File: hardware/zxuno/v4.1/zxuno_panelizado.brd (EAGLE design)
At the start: 190 x 150 mm, 414 parts, among them T1 BC846, T2 BC846, T3 BC846, T4 BC846, U1 6SLX9TQG144, U10 FLASH-SPI-25XXSMD1, U11 3.3V, U12 1.2V, U13 AD724, U14 50MHz, U15 6SLX9TQG144, U17 FLASH-SPI-25XXSMD1, U18 3.3V, U19 1.2V, U2 FLASH-SPI-25XXSMD1, U20 AD724, U21 50MHz, U22 6SLX9TQG144, U24 FLASH-SPI-25XXSMD1, U25 3.3V, U26 1.2V, U27 AD724, U28 50MHz, U4 AD724, U5 50MHz, U6 3.3V, U7 1.2V, U8 6SLX9TQG144, Y1 3.58M, Y2 4.43M, Y3 3.58M, Y4 4.43M, Y5 3.58M, Y6 4.43M, Y7 3.58M, Y8 4.43M

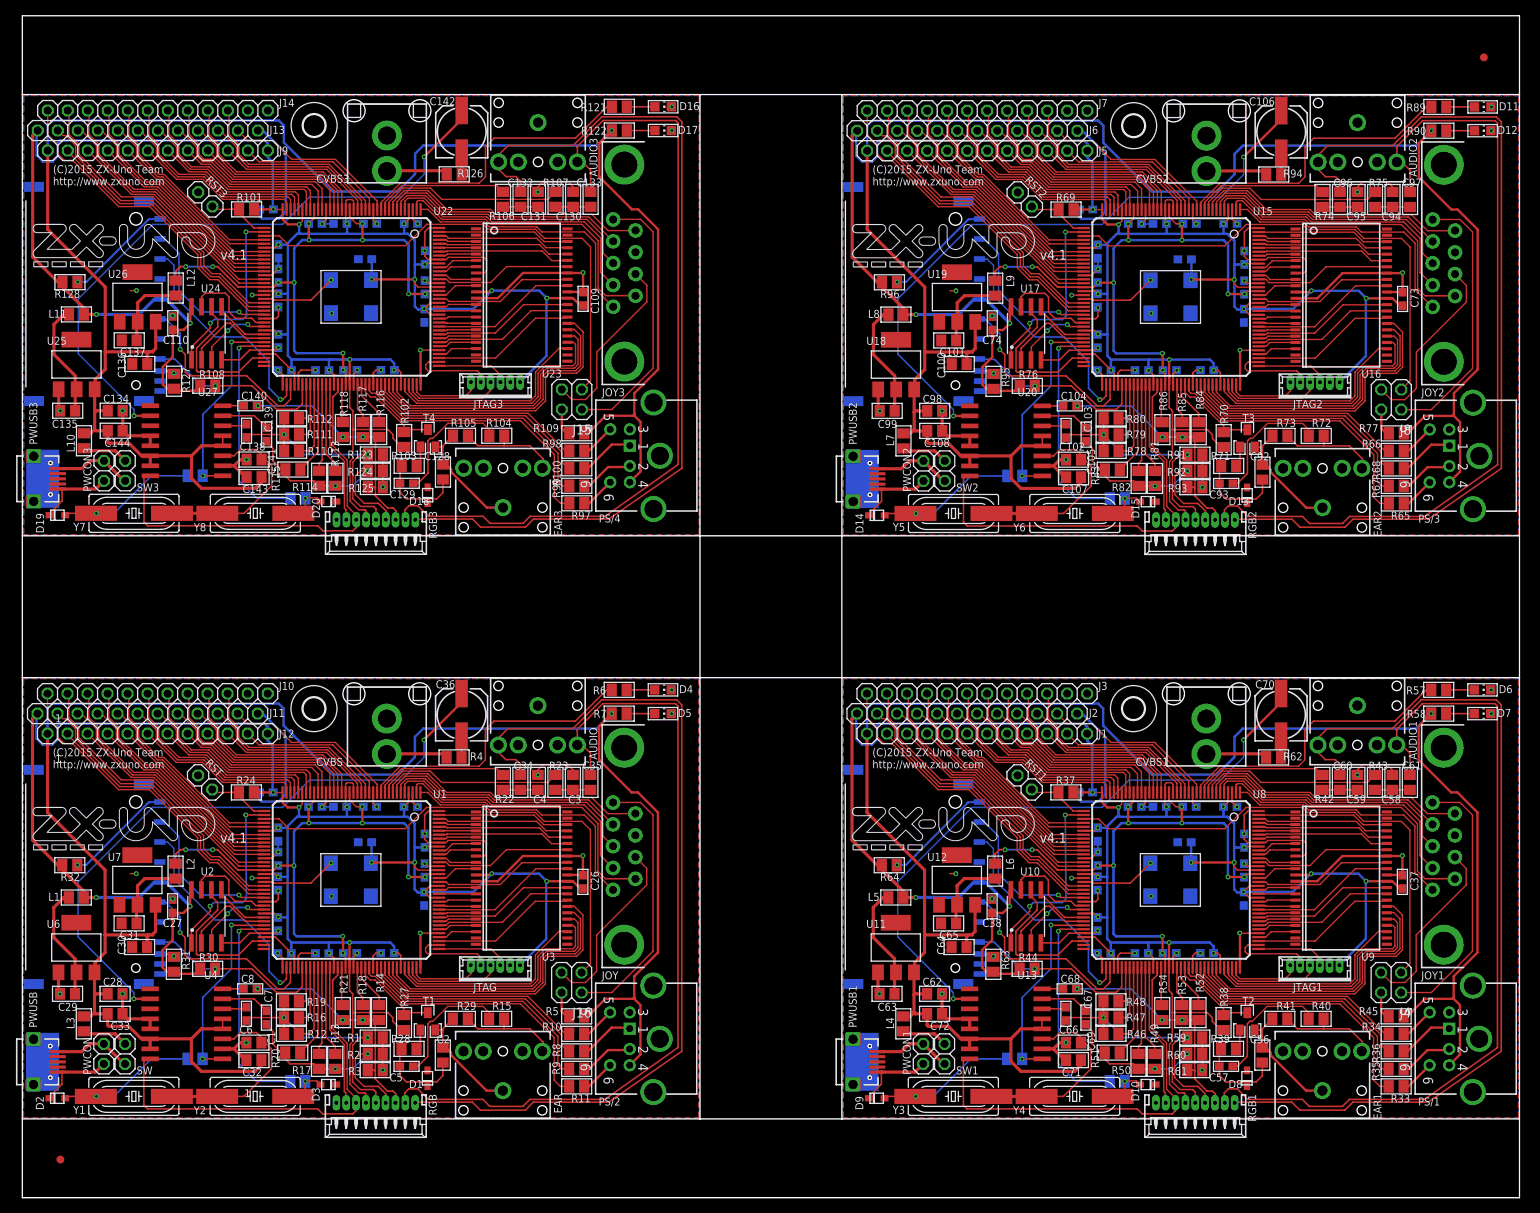
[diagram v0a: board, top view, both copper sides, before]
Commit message: Vacío panelizado
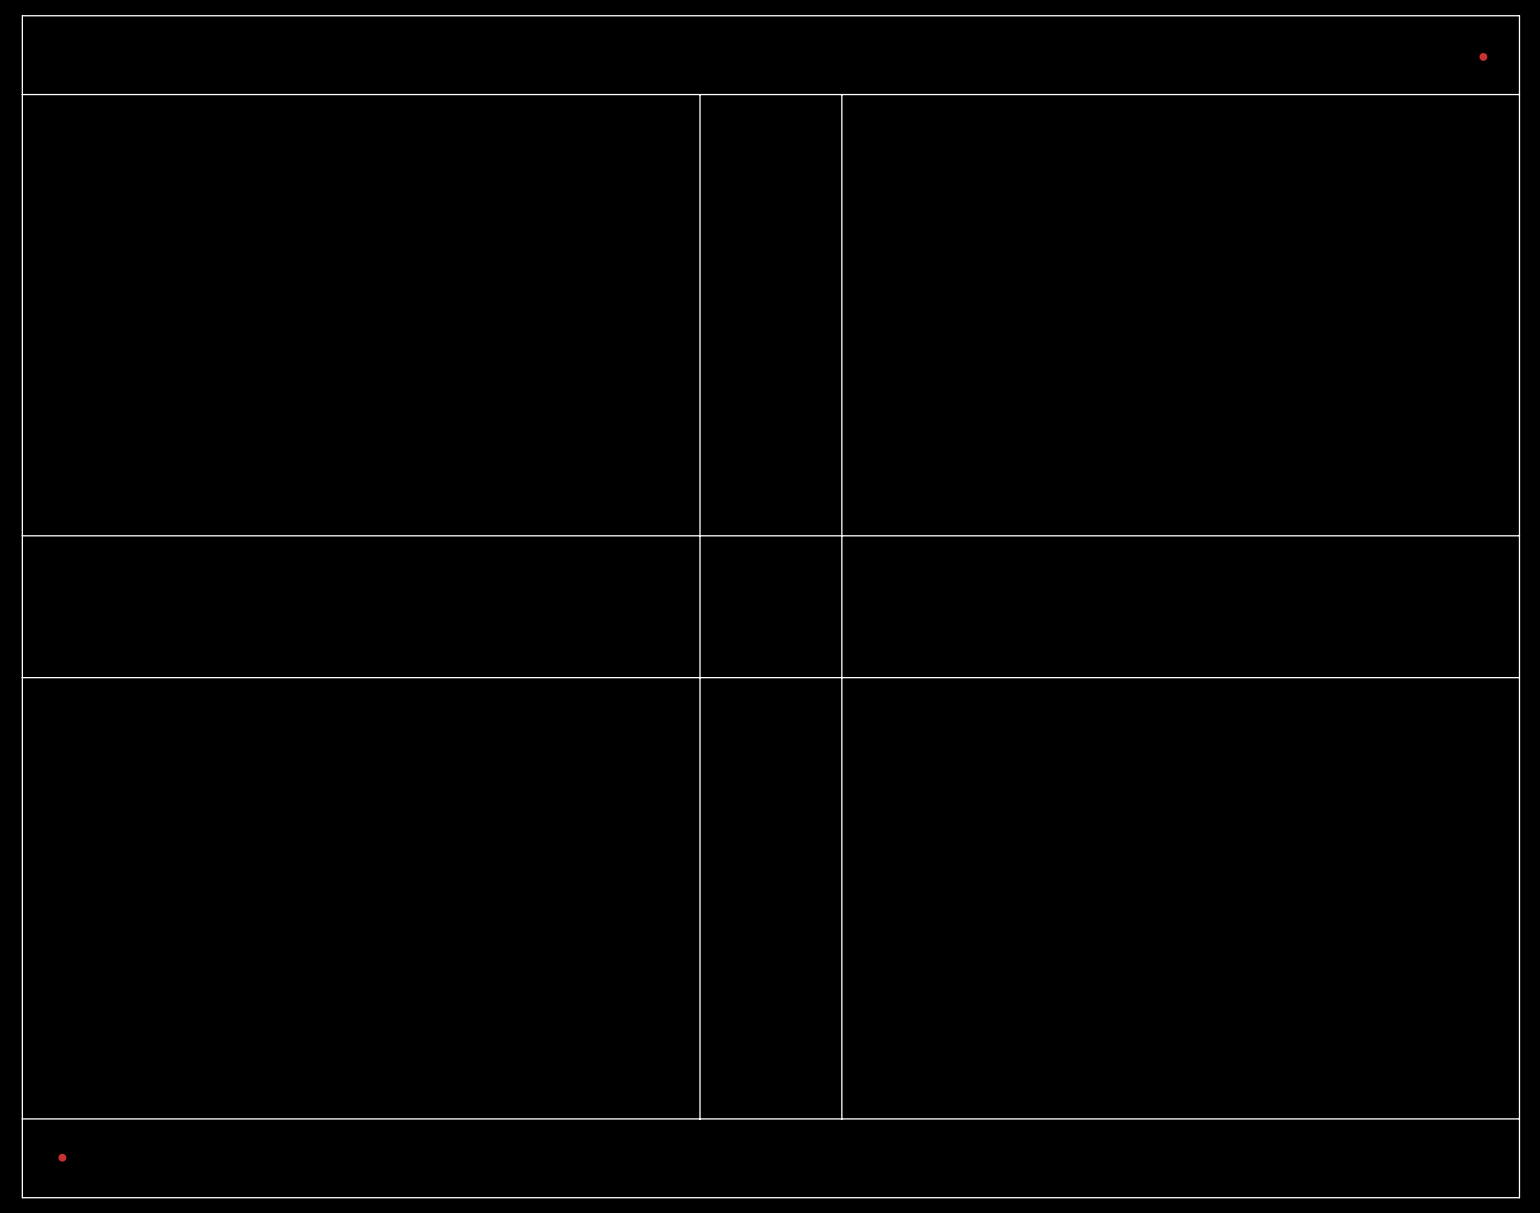
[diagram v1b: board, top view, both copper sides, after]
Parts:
- removed AUDIO, AUDIO1, AUDIO2, AUDIO3: Audio, SparkFun-Connectors:AUDIO-JACK
- removed C1, C105, C141, C69: 7.5pF, rcl:C0805
- removed C10, C102, C103, C104, C109, C11, C110, C111, C112, C113, C114, C115, C116, C117, C118, C119, C12, C120, C121, C122, C123, C124, C125, C126, C127, C129, C13, C138, C139, C14, C140, C15, C16, C17, C18, C19, C20, C21, C22, C23, C24, C25, C26, C27, C37, C38, C39, C40, C41, C42, C43, C44, C45, C46, C47, C48, C49, C5, C50, C51, C52, C53, C54, C55, C57, C6, C66, C67, C68, C7, C73, C74, C75, C76, C77, C78, C79, C8, C80, C81, C82, C83, C84, C85, C86, C87, C88, C89, C9, C90, C91, C93: 100nF, rcl:C0603
- removed C100, C101, C107, C108, C132, C133, C134, C135, C136, C137, C143, C144, C28, C29, C30, C31, C32, C33, C34, C35, C60, C61, C62, C63, C64, C65, C71, C72, C96, C97, C98, C99: 10uF, rcl:C0805
- removed C106, C142, C36, C70: 220uF, rcl:153CLV-0605
- removed C128, C130, C131, C2, C3, C4, C56, C58, C59, C92, C94, C95: 10nF, rcl:C0805
- removed CVBS, CVBS1, CVBS2, CVBS3: RCA, uzebox:RCA
- removed D1, D10, D13, D14, D15, D18, D19, D2, D20, D3, D8, D9: (no value), adafruit:SOD-323F
- removed D11, D12, D16, D17, D4, D5, D6, D7: (no value), led:CHIP-LED0805
- removed EAR, EAR1, EAR2, EAR3: EAR, SparkFun-Connectors:AUDIO-JACK
- removed H1, H2, H3, H4: MOUNT-HOLE2.8, holes:2,8
- removed J1, J10, J11, J12, J13, J14, J2, J3, J5, J6, J7, J9: (no value), pinhead:1X12
- removed J15, J16, J4, J8: (no value), pinhead:2X02
- removed JOY, JOY1, JOY2, JOY3: (no value), SparkFun-Connectors:DB9_MALE
- removed JTAG, JTAG1, JTAG2, JTAG3: JTAG, con-molex:53047-06
- removed L1, L10, L11, L12, L2, L3, L4, L5, L6, L7, L8, L9: (no value), rcl:M0805
- removed PS/1, PS/2, PS/3, PS/4: PS/2 Keyb, ZX_UNO_0_14:DINC/MIN_TM/6_1PRIMARY
- removed PWCON, PWCON1, PWCON2, PWCON3, RST, RST1, RST2, RST3, SW, SW1, SW2, SW3: (no value), pinhead:1X02
- removed PWUSB, PWUSB1, PWUSB2, PWUSB3: MICROUSB, zxuno_rev_mcleod:MICRO_USB_1PRIMARY
- removed R1, R123, R124, R125, R126, R2, R3, R4, R59, R60, R61, R62, R91, R92, R93, R94: 75, rcl:M0805
- removed R10, R100, R104, R109, R11, R110, R113, R116, R12, R121, R122, R13, R14, R15, R33, R34, R35, R36, R40, R45, R46, R49, R5, R52, R57, R58, R6, R65, R66, R67, R68, R7, R72, R77, R78, R8, R81, R84, R89, R9, R90, R97, R98, R99: 510, rcl:M0805
- removed R101, R106, R107, R112, R115, R118, R19, R20, R21, R22, R23, R24, R37, R42, R43, R48, R51, R54, R69, R74, R75, R80, R83, R86: 2K, rcl:M0805
- removed R102, R103, R105, R108, R119, R120, R127, R128, R25, R26, R27, R28, R29, R30, R31, R32, R38, R39, R41, R44, R55, R56, R63, R64, R70, R71, R73, R76, R87, R88, R95, R96: 10K, rcl:M0805
- removed R111, R114, R117, R16, R17, R18, R47, R50, R53, R79, R82, R85: 1K, rcl:M0805
- removed RGB, RGB1, RGB2, RGB3: RGB, con-molex:53048-09
- removed SDCARD, SDCARD1, SDCARD2, SDCARD3: (no value), zxuno_rev_mcleod:SDCMF-10915W010
- removed T1, T2, T3, T4: BC846, transistor:SOT23
- removed U1, U15, U22, U8: 6SLX9TQG144, xilinx_devices_V6:TQ144
- removed U10, U17, U2, U24: FLASH-SPI-25XXSMD1, GadgetFactory:SO08-EIAJ
- removed U11, U18, U25, U6: 3.3V, burr-brown:SOT223
- removed U12, U19, U26, U7: 1.2V, burr-brown:SOT223
- removed U13, U20, U27, U4: AD724, ad725:SO16W
- removed U14, U21, U28, U5: 50MHz, ZX_UNO_0_15:SM/OSC_1PRIMARY
- removed U16, U23, U3, U9: (no value), GadgetFactory:TSOP44-II
- removed Y1, Y3, Y5, Y7: 3.58M, crystal:HC49UP
- removed Y2, Y4, Y6, Y8: 4.43M, crystal:HC49UP
- moved E$1 0.35 mm to (5.08, 5.08)
- moved E$2 0.08 mm to (185.4, 144.8)
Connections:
- removed net 1.2V: C10.2, C11.2, C12.2, C13.2, C9.2, L2.2, U1.P128, U1.P19, U1.P28, U1.P52, U1.P89
- removed net 1.2V1: C39.2, C40.2, C41.2, C42.2, C43.2, L6.2, U8.P128, U8.P19, U8.P28, U8.P52, U8.P89
- removed net 1.2V2: C75.2, C76.2, C77.2, C78.2, C79.2, L9.2, U15.P128, U15.P19, U15.P28, U15.P52, U15.P89
- removed net 1.2V3: C111.2, C112.2, C113.2, C114.2, C115.2, L12.2, U22.P128, U22.P19, U22.P28, U22.P52, U22.P89
- removed net 3.3V: C14.2, C15.2, C16.2, C17.2, C18.2, C19.2, C20.2, C21.2, C22.2, C23.2, C24.2, C25.2, C26.1, C27.2, J11.1, J12.12, JTAG.1, L1.2, R24.2, R27.2, R30.1, R31.2, R32.2, RGB.4, SDCARD.4, U1.P103, U1.P122, U1.P125, U1.P129, U1.P135, U1.P18, U1.P20, U1.P31, U1.P36, U1.P4, U1.P42, U1.P53, U1.P63, U1.P69, U1.P76, U1.P86, U1.P90, U2.8, U3.11, U3.33, U5.4
- removed net 3.3V1: C37.1, C38.2, C44.2, C45.2, C46.2, C47.2, C48.2, C49.2, C50.2, C51.2, C52.2, C53.2, C54.2, C55.2, J1.12, J2.1, JTAG1.1, L5.2, R37.2, R38.2, R44.1, R63.2, R64.2, RGB1.4, SDCARD1.4, U10.8, U14.4, U8.P103, U8.P122, U8.P125, U8.P129, U8.P135, U8.P18, U8.P20, U8.P31, U8.P36, U8.P4, U8.P42, U8.P53, U8.P63, U8.P69, U8.P76, U8.P86, U8.P90, U9.11, U9.33
- removed net 3.3V2: C73.1, C74.2, C80.2, C81.2, C82.2, C83.2, C84.2, C85.2, C86.2, C87.2, C88.2, C89.2, C90.2, C91.2, J5.12, J6.1, JTAG2.1, L8.2, R69.2, R70.2, R76.1, R95.2, R96.2, RGB2.4, SDCARD2.4, U15.P103, U15.P122, U15.P125, U15.P129, U15.P135, U15.P18, U15.P20, U15.P31, U15.P36, U15.P4, U15.P42, U15.P53, U15.P63, U15.P69, U15.P76, U15.P86, U15.P90, U16.11, U16.33, U17.8, U21.4
- removed net 3.3V3: C109.1, C110.2, C116.2, C117.2, C118.2, C119.2, C120.2, C121.2, C122.2, C123.2, C124.2, C125.2, C126.2, C127.2, J13.1, J9.12, JTAG3.1, L11.2, R101.2, R102.2, R108.1, R127.2, R128.2, RGB3.4, SDCARD3.4, U22.P103, U22.P122, U22.P125, U22.P129, U22.P135, U22.P18, U22.P20, U22.P31, U22.P36, U22.P4, U22.P42, U22.P53, U22.P63, U22.P69, U22.P76, U22.P86, U22.P90, U23.11, U23.33, U24.8, U28.4
- removed net 5V: C28.1, C30.1, C32.2, C33.2, J12.1, L3.2, PS/2.4, R5.1, R7.2, U4.14, U4.15, U4.4, U4.5, U6.3, U7.3
- removed net 5V1: C62.1, C64.1, C71.2, C72.2, J1.1, L4.2, PS/1.4, R45.1, R58.2, U11.3, U12.3, U13.14, U13.15, U13.4, U13.5
- removed net 5V2: C100.1, C107.2, C108.2, C98.1, J5.1, L7.2, PS/3.4, R77.1, R90.2, U18.3, U19.3, U20.14, U20.15, U20.4, U20.5
- removed net 5V3: C134.1, C136.1, C143.2, C144.2, J9.1, L10.2, PS/4.4, R109.1, R122.2, U25.3, U26.3, U27.14, U27.15, U27.4, U27.5
- removed net AUDIO_LEFT: R22.2, U1.P10
- removed net AUDIO_LEFT1: R42.2, U8.P10
- removed net AUDIO_LEFT2: R74.2, U15.P10
- removed net AUDIO_LEFT3: R106.2, U22.P10
- removed net AUDIO_RIGHT: R23.2, U1.P9
- removed net AUDIO_RIGHT1: R43.2, U8.P9
- removed net AUDIO_RIGHT2: R75.2, U15.P9
- removed net AUDIO_RIGHT3: R107.2, U22.P9
- removed net B: C8.2, R14.1, R18.1, R21.1, R3.1, RGB.7
- removed net B0: R21.2, U1.P88
- removed net B1: R18.2, U1.P92
- removed net B10: C104.2, R84.1, R85.1, R86.1, R93.1, RGB2.7
- removed net B11: R118.2, U22.P88
- removed net B12: R117.2, U22.P92
- removed net B13: R116.2, U22.P93
- removed net B14: C140.2, R116.1, R117.1, R118.1, R125.1, RGB3.7
- removed net B2: R14.2, U1.P93
- removed net B3: R54.2, U8.P88
- removed net B4: R53.2, U8.P92
- removed net B5: R52.2, U8.P93
- removed net B6: C68.2, R52.1, R53.1, R54.1, R61.1, RGB1.7
- removed net B7: R86.2, U15.P88
- removed net B8: R85.2, U15.P92
- removed net B9: R84.2, U15.P93
- removed net CLK: U1.P55, U5.3
- removed net CLK1: U14.3, U8.P55
- removed net CLK2: U15.P55, U21.3
- removed net CLK3: U22.P55, U28.3
- removed net CSYNC: RGB.3, U1.P87, U4.16
- removed net CSYNC1: RGB1.3, U13.16, U8.P87
- removed net CSYNC2: RGB2.3, U15.P87, U20.16
- removed net CSYNC3: RGB3.3, U22.P87, U27.16
- removed net EAR: R27.1, T1.3, U1.P94
- removed net EAR1: R38.1, T2.3, U8.P94
- removed net EAR2: R70.1, T3.3, U15.P94
- removed net EAR3: R102.1, T4.3, U22.P94
- removed net EXT1: J1.2, U8.P57
- removed net EXT10: J12.3, U1.P50
- removed net EXT100: J9.5, U22.P43
- removed net EXT101: J13.5, U22.P41
- removed net EXT102: J14.5, U22.P40
- removed net EXT103: J9.6, U22.P35
- removed net EXT104: J13.6, U22.P34
- removed net EXT105: J14.6, U22.P33
- removed net EXT106: J9.7, U22.P32
- removed net EXT107: J13.7, U22.P30
- removed net EXT108: J14.7, U22.P29
- removed net EXT109: J9.8, U22.P27
- removed net EXT11: J11.3, U1.P48
- removed net EXT110: J13.8, U22.P26
- removed net EXT111: J14.8, U22.P24
- removed net EXT112: J9.9, U22.P23
- removed net EXT113: J13.9, U22.P22
- removed net EXT114: J14.9, U22.P21
- removed net EXT115: J9.10, U22.P17
- removed net EXT116: J13.10, U22.P16
- removed net EXT117: J14.10, U22.P15
- removed net EXT118: J9.11, U22.P14
- removed net EXT119: J13.11, U22.P12
- removed net EXT12: J10.3, U1.P47
- removed net EXT120: J14.1, U22.P58
- removed net EXT13: J12.4, U1.P46
- removed net EXT14: J11.4, U1.P45
- removed net EXT15: J10.4, U1.P44
- removed net EXT16: J12.5, U1.P43
- removed net EXT17: J11.5, U1.P41
- removed net EXT18: J10.5, U1.P40
- removed net EXT19: J12.6, U1.P35
- removed net EXT2: J2.2, U8.P56
- removed net EXT20: J11.6, U1.P34
- removed net EXT21: J10.6, U1.P33
- removed net EXT22: J12.7, U1.P32
- removed net EXT23: J11.7, U1.P30
- removed net EXT24: J10.7, U1.P29
- removed net EXT25: J12.8, U1.P27
- removed net EXT26: J11.8, U1.P26
- removed net EXT27: J10.8, U1.P24
- removed net EXT28: J12.9, U1.P23
- removed net EXT29: J11.9, U1.P22
- removed net EXT3: J3.2, U8.P51
- removed net EXT30: J10.9, U1.P21
- removed net EXT31: J12.10, U1.P17
- removed net EXT32: J11.10, U1.P16
- removed net EXT33: J10.10, U1.P15
- removed net EXT34: J12.11, U1.P14
- removed net EXT35: J11.11, U1.P12
- removed net EXT36: J3.3, U8.P47
- removed net EXT37: J1.4, U8.P46
- removed net EXT38: J2.4, U8.P45
- removed net EXT39: J3.4, U8.P44
- removed net EXT4: J1.3, U8.P50
- removed net EXT40: J1.5, U8.P43
- removed net EXT41: J2.5, U8.P41
- removed net EXT42: J3.5, U8.P40
- removed net EXT43: J1.6, U8.P35
- removed net EXT44: J2.6, U8.P34
- removed net EXT45: J3.6, U8.P33
- removed net EXT46: J1.7, U8.P32
- removed net EXT47: J2.7, U8.P30
- removed net EXT48: J3.7, U8.P29
- removed net EXT49: J1.8, U8.P27
- removed net EXT5: J2.3, U8.P48
- removed net EXT50: J2.8, U8.P26
- removed net EXT51: J3.8, U8.P24
- removed net EXT52: J1.9, U8.P23
- removed net EXT53: J2.9, U8.P22
- removed net EXT54: J3.9, U8.P21
- removed net EXT55: J1.10, U8.P17
- removed net EXT56: J2.10, U8.P16
- removed net EXT57: J3.10, U8.P15
- removed net EXT58: J1.11, U8.P14
- removed net EXT59: J2.11, U8.P12
- removed net EXT6: J10.1, U1.P58
- removed net EXT60: J3.1, U8.P58
- removed net EXT61: J5.2, U15.P57
- removed net EXT62: J6.2, U15.P56
- removed net EXT63: J7.2, U15.P51
- removed net EXT64: J5.3, U15.P50
- removed net EXT65: J6.3, U15.P48
- removed net EXT66: J7.3, U15.P47
- removed net EXT67: J5.4, U15.P46
- removed net EXT68: J6.4, U15.P45
- removed net EXT69: J7.4, U15.P44
- removed net EXT7: J12.2, U1.P57
- removed net EXT70: J5.5, U15.P43
- removed net EXT71: J6.5, U15.P41
- removed net EXT72: J7.5, U15.P40
- removed net EXT73: J5.6, U15.P35
- removed net EXT74: J6.6, U15.P34
- removed net EXT75: J7.6, U15.P33
- removed net EXT76: J5.7, U15.P32
- removed net EXT77: J6.7, U15.P30
- removed net EXT78: J7.7, U15.P29
- removed net EXT79: J5.8, U15.P27
- removed net EXT8: J11.2, U1.P56
- removed net EXT80: J6.8, U15.P26
- removed net EXT81: J7.8, U15.P24
- removed net EXT82: J5.9, U15.P23
- removed net EXT83: J6.9, U15.P22
- removed net EXT84: J7.9, U15.P21
- removed net EXT85: J5.10, U15.P17
- removed net EXT86: J6.10, U15.P16
- removed net EXT87: J7.10, U15.P15
- removed net EXT88: J5.11, U15.P14
- removed net EXT89: J6.11, U15.P12
- removed net EXT9: J10.2, U1.P51
- removed net EXT90: J7.1, U15.P58
- removed net EXT91: J9.2, U22.P57
- removed net EXT92: J13.2, U22.P56
- removed net EXT93: J14.2, U22.P51
- removed net EXT94: J9.3, U22.P50
- removed net EXT95: J13.3, U22.P48
- removed net EXT96: J14.3, U22.P47
- removed net EXT97: J9.4, U22.P46
- removed net EXT98: J13.4, U22.P45
- removed net EXT99: J14.4, U22.P44
- removed net FLASH_CS: U1.P38, U2.1
- removed net FLASH_CS1: U10.1, U8.P38
- removed net FLASH_CS2: U15.P38, U17.1
- removed net FLASH_CS3: U22.P38, U24.1
- removed net FLASH_HOLD: U1.P61, U2.7
- removed net FLASH_HOLD1: U10.7, U8.P61
- removed net FLASH_HOLD2: U15.P61, U17.7
- removed net FLASH_HOLD3: U22.P61, U24.7
- removed net FLASH_MISO: U1.P65, U2.2
- removed net FLASH_MISO1: U10.2, U8.P65
- removed net FLASH_MISO2: U15.P65, U17.2
- removed net FLASH_MISO3: U22.P65, U24.2
- removed net FLASH_MOSI: U1.P64, U2.5
- removed net FLASH_MOSI1: U10.5, U8.P64
- removed net FLASH_MOSI2: U15.P64, U17.5
- removed net FLASH_MOSI3: U22.P64, U24.5
- removed net FLASH_SCK: U1.P70, U2.6
- removed net FLASH_SCK1: U10.6, U8.P70
- removed net FLASH_SCK2: U15.P70, U17.6
- removed net FLASH_SCK3: U22.P70, U24.6
- removed net FLASH_WP: U1.P62, U2.3
- removed net FLASH_WP1: U10.3, U8.P62
- removed net FLASH_WP2: U15.P62, U17.3
- removed net FLASH_WP3: U22.P62, U24.3
- removed net G: C7.2, R13.1, R17.1, R2.1, R20.1, RGB.6
- removed net G0: R20.2, U1.P82
- removed net G1: R17.2, U1.P83
- removed net G10: C103.2, R81.1, R82.1, R83.1, R92.1, RGB2.6
- removed net G11: R115.2, U22.P82
- removed net G12: R114.2, U22.P83
- removed net G13: R113.2, U22.P84
- removed net G14: C139.2, R113.1, R114.1, R115.1, R124.1, RGB3.6
- removed net G2: R13.2, U1.P84
- removed net G3: R51.2, U8.P82
- removed net G4: R50.2, U8.P83
- removed net G5: R49.2, U8.P84
- removed net G6: C67.2, R49.1, R50.1, R51.1, R60.1, RGB1.6
- removed net G7: R83.2, U15.P82
- removed net G8: R82.2, U15.P83
- removed net G9: R81.2, U15.P84
- removed net GND: AUDIO.SLEEVE, C1.2, C10.1, C11.1, C12.1, C13.1, C14.1, C15.1, C16.1, C17.1, C18.1, C19.1, C2.2, C20.1, C21.1, C22.1, C23.1, C24.1, C25.1, C26.2, C27.1, C28.2, C29.2, C3.2, C30.2, C31.2, C32.1, C33.1, C4.2, C9.1, CVBS.GND, D1.A, D2.C, D3.C, D4.C, D5.C, EAR.SLEEVE, J10.12, J11.12, JOY.8, JTAG.2, PS/2.3, PWCON.1, PWUSB.5, R1.2, R2.2, R29.2, R3.2, RGB.1, RST.1, SDCARD.3, SDCARD.6, SDCARD.M1, SDCARD.M2, SDCARD.M3, SDCARD.M4, T1.2, U1.P108, U1.P113, U1.P13, U1.P130, U1.P136, U1.P144, U1.P25, U1.P3, U1.P49, U1.P54, U1.P60, U1.P68, U1.P73, U1.P77, U1.P91, U1.P96, U2.4, U3.12, U3.34, U3.37, U3.8, U4.12, U4.13, U4.2, U5.2, U6.1, U7.1
- removed net GND1: AUDIO1.SLEEVE, C37.2, C38.1, C39.1, C40.1, C41.1, C42.1, C43.1, C44.1, C45.1, C46.1, C47.1, C48.1, C49.1, C50.1, C51.1, C52.1, C53.1, C54.1, C55.1, C56.2, C58.2, C59.2, C62.2, C63.2, C64.2, C65.2, C69.2, C71.1, C72.1, CVBS1.GND, D10.C, D6.C, D7.C, D8.A, D9.C, EAR1.SLEEVE, J2.12, J3.12, JOY1.8, JTAG1.2, PS/1.3, PWCON1.1, PWUSB1.5, R41.2, R59.2, R60.2, R61.2, RGB1.1, RST1.1, SDCARD1.3, SDCARD1.6, SDCARD1.M1, SDCARD1.M2, SDCARD1.M3, SDCARD1.M4, T2.2, U10.4, U11.1, U12.1, U13.12, U13.13, U13.2, U14.2, U8.P108, U8.P113, U8.P13, U8.P130, U8.P136, U8.P144, U8.P25, U8.P3, U8.P49, U8.P54, U8.P60, U8.P68, U8.P73, U8.P77, U8.P91, U8.P96, U9.12, U9.34, U9.37, U9.8
- removed net GND2: AUDIO2.SLEEVE, C100.2, C101.2, C105.2, C107.1, C108.1, C73.2, C74.1, C75.1, C76.1, C77.1, C78.1, C79.1, C80.1, C81.1, C82.1, C83.1, C84.1, C85.1, C86.1, C87.1, C88.1, C89.1, C90.1, C91.1, C92.2, C94.2, C95.2, C98.2, C99.2, CVBS2.GND, D11.C, D12.C, D13.A, D14.C, D15.C, EAR2.SLEEVE, J6.12, J7.12, JOY2.8, JTAG2.2, PS/3.3, PWCON2.1, PWUSB2.5, R73.2, R91.2, R92.2, R93.2, RGB2.1, RST2.1, SDCARD2.3, SDCARD2.6, SDCARD2.M1, SDCARD2.M2, SDCARD2.M3, SDCARD2.M4, T3.2, U15.P108, U15.P113, U15.P13, U15.P130, U15.P136, U15.P144, U15.P25, U15.P3, U15.P49, U15.P54, U15.P60, U15.P68, U15.P73, U15.P77, U15.P91, U15.P96, U16.12, U16.34, U16.37, U16.8, U17.4, U18.1, U19.1, U20.12, U20.13, U20.2, U21.2
- removed net GND3: AUDIO3.SLEEVE, C109.2, C110.1, C111.1, C112.1, C113.1, C114.1, C115.1, C116.1, C117.1, C118.1, C119.1, C120.1, C121.1, C122.1, C123.1, C124.1, C125.1, C126.1, C127.1, C128.2, C130.2, C131.2, C134.2, C135.2, C136.2, C137.2, C141.2, C143.1, C144.1, CVBS3.GND, D16.C, D17.C, D18.A, D19.C, D20.C, EAR3.SLEEVE, J13.12, J14.12, JOY3.8, JTAG3.2, PS/4.3, PWCON3.1, PWUSB3.5, R105.2, R123.2, R124.2, R125.2, RGB3.1, RST3.1, SDCARD3.3, SDCARD3.6, SDCARD3.M1, SDCARD3.M2, SDCARD3.M3, SDCARD3.M4, T4.2, U22.P108, U22.P113, U22.P13, U22.P130, U22.P136, U22.P144, U22.P25, U22.P3, U22.P49, U22.P54, U22.P60, U22.P68, U22.P73, U22.P77, U22.P91, U22.P96, U23.12, U23.34, U23.37, U23.8, U24.4, U25.1, U26.1, U27.12, U27.13, U27.2, U28.2
- removed net JOY_DOWN: JOY.2, U1.P5
- removed net JOY_DOWN1: JOY1.2, U8.P5
- removed net JOY_DOWN2: JOY2.2, U15.P5
- removed net JOY_DOWN3: JOY3.2, U22.P5
- removed net JOY_FIRE1: JOY.6, U1.P2
- removed net JOY_FIRE10: JOY3.6, U22.P2
- removed net JOY_FIRE11: JOY3.9, U22.P8
- removed net JOY_FIRE12: J15.1, U22.P39
- removed net JOY_FIRE2: JOY.9, U1.P8
- removed net JOY_FIRE3: J16.1, U1.P39
- removed net JOY_FIRE4: JOY1.6, U8.P2
- removed net JOY_FIRE5: JOY1.9, U8.P8
- removed net JOY_FIRE6: J4.1, U8.P39
- removed net JOY_FIRE7: JOY2.6, U15.P2
- removed net JOY_FIRE8: JOY2.9, U15.P8
- removed net JOY_FIRE9: J8.1, U15.P39
- removed net JOY_LEFT: JOY.3, U1.P6
- removed net JOY_LEFT1: JOY1.3, U8.P6
- removed net JOY_LEFT2: JOY2.3, U15.P6
- removed net JOY_LEFT3: JOY3.3, U22.P6
- removed net JOY_RIGHT: JOY.4, U1.P7
- removed net JOY_RIGHT1: JOY1.4, U8.P7
- removed net JOY_RIGHT2: JOY2.4, U15.P7
- removed net JOY_RIGHT3: JOY3.4, U22.P7
- removed net JOY_UP: JOY.1, U1.P1
- removed net JOY_UP1: JOY1.1, U8.P1
- removed net JOY_UP2: JOY2.1, U15.P1
- removed net JOY_UP3: JOY3.1, U22.P1
- removed net L-OUT: AUDIO.TIP, C34.2, RGB.9
- removed net L-OUT1: AUDIO1.TIP, C60.2, RGB1.9
- removed net L-OUT2: AUDIO2.TIP, C96.2, RGB2.9
- removed net L-OUT3: AUDIO3.TIP, C132.2, RGB3.9
- removed net LED: R6.2, U1.P11
- removed net LED1: R57.2, U8.P11
- removed net LED2: R89.2, U15.P11
- removed net LED3: R121.2, U22.P11
- removed net N$1: PS/2.6, R11.1
- removed net N$10: C3.1, C35.1, R23.1
- removed net N$100: C135.1, L11.1, U25.2
- removed net N$101: C137.1, L12.1, U26.2
- removed net N$102: C139.1, U27.7
- removed net N$103: C138.1, U27.6
- removed net N$104: C141.1, U27.3, Y7.2, Y8.2
- removed net N$105: D20.A, R120.1, Y8.1
- removed net N$106: D19.A, R119.2, Y7.1
- removed net N$107: C142.+, U27.10
- removed net N$108: C140.1, U27.8
- removed net N$109: C142.-, R126.1
- removed net N$11: C34.1, C4.1, R22.1
- removed net N$110: CVBS3.SIG, R126.2
- removed net N$111: D16.A, R121.1
- removed net N$112: D17.A, R122.1
- removed net N$113: R101.1, RST3.2, U22.P37
- removed net N$114: R127.1, SDCARD3.8
- removed net N$115: R128.1, SDCARD3.9
- removed net N$116: J15.4, R109.2
- removed net N$12: PWCON.2, PWUSB.1, SW.2
- removed net N$13: L3.1, SW.1
- removed net N$14: C29.1, L1.1, U6.2
- removed net N$15: J16.4, R5.2
- removed net N$16: PS/1.6, R33.1
- removed net N$17: C31.1, L2.1, U7.2
- removed net N$18: R31.1, SDCARD.8
- removed net N$19: C8.1, U4.8
- removed net N$2: PS/2.5, R10.1
- removed net N$20: R32.1, SDCARD.9
- removed net N$21: C7.1, U4.7
- removed net N$22: C6.1, U4.6
- removed net N$23: C1.1, U4.3, Y1.2, Y2.2
- removed net N$24: D3.A, R26.1, Y2.1
- removed net N$25: D2.A, R25.2, Y1.1
- removed net N$26: C36.+, U4.10
- removed net N$27: C36.-, R4.1
- removed net N$28: CVBS.SIG, R4.2
- removed net N$29: PS/1.5, R34.1
- removed net N$3: PS/2.2, R9.1
- removed net N$30: PS/1.2, R35.1
- removed net N$31: D4.A, R6.1
- removed net N$32: D5.A, R7.1
- removed net N$33: PS/1.1, R36.1
- removed net N$34: R39.2, T2.1
- removed net N$35: C56.1, C57.1, D8.C, R39.1
- removed net N$36: C57.2, R40.2
- removed net N$37: EAR1.TIP, R40.1, R41.1
- removed net N$38: C58.1, C61.1, R43.1
- removed net N$39: C59.1, C60.1, R42.1
- removed net N$4: PS/2.1, R8.1
- removed net N$40: PWCON1.2, PWUSB1.1, SW1.2
- removed net N$41: L4.1, SW1.1
- removed net N$42: C63.1, L5.1, U11.2
- removed net N$43: C65.1, L6.1, U12.2
- removed net N$44: C67.1, U13.7
- removed net N$45: C66.1, U13.6
- removed net N$46: C69.1, U13.3, Y3.2, Y4.2
- removed net N$47: D10.A, R56.1, Y4.1
- removed net N$48: D9.A, R55.2, Y3.1
- removed net N$49: C70.+, U13.10
- removed net N$5: R24.1, RST.2, U1.P37
- removed net N$50: C68.1, U13.8
- removed net N$51: C70.-, R62.1
- removed net N$52: CVBS1.SIG, R62.2
- removed net N$53: D6.A, R57.1
- removed net N$54: D7.A, R58.1
- removed net N$55: R37.1, RST1.2, U8.P37
- removed net N$56: R63.1, SDCARD1.8
- removed net N$57: R64.1, SDCARD1.9
- removed net N$58: J4.4, R45.2
- removed net N$59: PS/3.6, R65.1
- removed net N$6: R28.2, T1.1
- removed net N$60: PS/3.5, R66.1
- removed net N$61: PS/3.2, R67.1
- removed net N$62: PS/3.1, R68.1
- removed net N$63: R71.2, T3.1
- removed net N$64: C92.1, C93.1, D13.C, R71.1
- removed net N$65: C93.2, R72.2
- removed net N$66: EAR2.TIP, R72.1, R73.1
- removed net N$67: C94.1, C97.1, R75.1
- removed net N$68: C95.1, C96.1, R74.1
- removed net N$69: PWCON2.2, PWUSB2.1, SW2.2
- removed net N$7: C2.1, C5.1, D1.C, R28.1
- removed net N$70: L7.1, SW2.1
- removed net N$71: C99.1, L8.1, U18.2
- removed net N$72: C101.1, L9.1, U19.2
- removed net N$73: C103.1, U20.7
- removed net N$74: C102.1, U20.6
- removed net N$75: C105.1, U20.3, Y5.2, Y6.2
- removed net N$76: D15.A, R88.1, Y6.1
- removed net N$77: D14.A, R87.2, Y5.1
- removed net N$78: C106.+, U20.10
- removed net N$79: C104.1, U20.8
- removed net N$8: C5.2, R15.2
- removed net N$80: C106.-, R94.1
- removed net N$81: CVBS2.SIG, R94.2
- removed net N$82: D11.A, R89.1
- removed net N$83: D12.A, R90.1
- removed net N$84: R69.1, RST2.2, U15.P37
- removed net N$85: R95.1, SDCARD2.8
- removed net N$86: R96.1, SDCARD2.9
- removed net N$87: J8.4, R77.2
- removed net N$88: PS/4.6, R97.1
- removed net N$89: PS/4.5, R98.1
- removed net N$9: EAR.TIP, R15.1, R29.1
- removed net N$90: PS/4.2, R99.1
- removed net N$91: PS/4.1, R100.1
- removed net N$92: R103.2, T4.1
- removed net N$93: C128.1, C129.1, D18.C, R103.1
- removed net N$94: C129.2, R104.2
- removed net N$95: EAR3.TIP, R104.1, R105.1
- removed net N$96: C130.1, C133.1, R107.1
- removed net N$97: C131.1, C132.1, R106.1
- removed net N$98: PWCON3.2, PWUSB3.1, SW3.2
- removed net N$99: L10.1, SW3.1
- removed net PIN1: J4.3, JOY1.7
- removed net PIN2: J4.2, JOY1.5
- removed net PIN3: J8.3, JOY2.7
- removed net PIN4: J8.2, JOY2.5
- removed net PIN5: J16.2, JOY.5
- removed net PIN6: J15.3, JOY3.7
- removed net PIN7: J16.3, JOY.7
- removed net PIN8: J15.2, JOY3.5
- removed net PS2_CLK: R10.2, U1.P99
- removed net PS2_CLK1: R34.2, U8.P99
- removed net PS2_CLK2: R66.2, U15.P99
- removed net PS2_CLK3: R98.2, U22.P99
- removed net PS2_DATA: R8.2, U1.P98
- removed net PS2_DATA1: R36.2, U8.P98
- removed net PS2_DATA2: R68.2, U15.P98
- removed net PS2_DATA3: R100.2, U22.P98
- removed net PS2_PIN1: R33.2, U8.P95
- removed net PS2_PIN2: R9.2, U1.P97
- removed net PS2_PIN3: R35.2, U8.P97
- removed net PS2_PIN4: R65.2, U15.P95
- removed net PS2_PIN5: R67.2, U15.P97
- removed net PS2_PIN6: R11.2, U1.P95
- removed net PS2_PIN7: R97.2, U22.P95
- removed net PS2_PIN8: R99.2, U22.P97
- removed net R: C6.2, R1.1, R12.1, R16.1, R19.1, RGB.5
- removed net R-OUT: AUDIO.RING, C35.2, RGB.8
- removed net R-OUT1: AUDIO1.RING, C61.2, RGB1.8
- removed net R-OUT2: AUDIO2.RING, C97.2, RGB2.8
- removed net R-OUT3: AUDIO3.RING, C133.2, RGB3.8
- removed net R0: R19.2, U1.P79
- removed net R1: R16.2, U1.P80
- removed net R10: C102.2, R78.1, R79.1, R80.1, R91.1, RGB2.5
- removed net R11: R112.2, U22.P79
- removed net R12: R111.2, U22.P80
- removed net R13: R110.2, U22.P81
- removed net R14: C138.2, R110.1, R111.1, R112.1, R123.1, RGB3.5
- removed net R2: R12.2, U1.P81
- removed net R3: R48.2, U8.P79
- removed net R4: R47.2, U8.P80
- removed net R5: R46.2, U8.P81
- removed net R6: C66.2, R46.1, R47.1, R48.1, R59.1, RGB1.5
- removed net R7: R80.2, U15.P79
- removed net R8: R79.2, U15.P80
- removed net R9: R78.2, U15.P81
- removed net SD_CS: SDCARD.1, U1.P59
- removed net SD_CS1: SDCARD1.1, U8.P59
- removed net SD_CS2: SDCARD2.1, U15.P59
- removed net SD_CS3: SDCARD3.1, U22.P59
- removed net SD_MISO: R30.2, SDCARD.7, U1.P78
- removed net SD_MISO1: R44.2, SDCARD1.7, U8.P78
- removed net SD_MISO2: R76.2, SDCARD2.7, U15.P78
- removed net SD_MISO3: R108.2, SDCARD3.7, U22.P78
- removed net SD_MOSI: SDCARD.2, U1.P74
- removed net SD_MOSI1: SDCARD1.2, U8.P74
- removed net SD_MOSI2: SDCARD2.2, U15.P74
- removed net SD_MOSI3: SDCARD3.2, U22.P74
- removed net SD_SCK: SDCARD.5, U1.P75
- removed net SD_SCK1: SDCARD1.5, U8.P75
- removed net SD_SCK2: SDCARD2.5, U15.P75
- removed net SD_SCK3: SDCARD3.5, U22.P75
- removed net STDN: R25.1, U1.P66, U4.1
- removed net STDN1: R55.1, U13.1, U8.P66
- removed net STDN2: R87.1, U15.P66, U20.1
- removed net STDN3: R119.1, U22.P66, U27.1
- removed net STDNB: R26.2, U1.P67
- removed net STDNB1: R56.2, U8.P67
- removed net STDNB2: R88.2, U15.P67
- removed net STDNB3: R120.2, U22.P67
- removed net TCK: JTAG.3, U1.P109
- removed net TCK1: JTAG1.3, U8.P109
- removed net TCK2: JTAG2.3, U15.P109
- removed net TCK3: JTAG3.3, U22.P109
- removed net TDI: JTAG.5, U1.P110
- removed net TDI1: JTAG1.5, U8.P110
- removed net TDI2: JTAG2.5, U15.P110
- removed net TDI3: JTAG3.5, U22.P110
- removed net TDO: JTAG.4, U1.P106
- removed net TDO1: JTAG1.4, U8.P106
- removed net TDO2: JTAG2.4, U15.P106
- removed net TDO3: JTAG3.4, U22.P106
- removed net TMS: JTAG.6, U1.P107
- removed net TMS1: JTAG1.6, U8.P107
- removed net TMS2: JTAG2.6, U15.P107
- removed net TMS3: JTAG3.6, U22.P107
- removed net VSYNC: RGB.2, U1.P85
- removed net VSYNC1: RGB1.2, U8.P85
- removed net VSYNC2: RGB2.2, U15.P85
- removed net VSYNC3: RGB3.2, U22.P85
- removed net WR: U1.P121, U3.15
- removed net WR1: U8.P121, U9.15
- removed net WR2: U15.P121, U16.15
- removed net WR3: U22.P121, U23.15
- removed net XA0: U1.P141, U3.3
- removed net XA1: U1.P139, U3.4
- removed net XA10: U1.P104, U3.26
- removed net XA11: U1.P102, U3.27
- removed net XA12: U1.P101, U3.28
- removed net XA13: U1.P100, U3.29
- removed net XA14: U1.P111, U3.30
- removed net XA15: U1.P131, U3.38
- removed net XA16: U1.P138, U3.39
- removed net XA17: U1.P140, U3.40
- removed net XA18: U1.P142, U3.41
- removed net XA19: U1.P105, U3.25
- removed net XA2: U1.P137, U3.5
- removed net XA20: U1.P143, U3.42
- removed net XA21: U8.P141, U9.3
- removed net XA22: U8.P137, U9.5
- removed net XA23: U8.P134, U9.6
- removed net XA24: U8.P133, U9.7
- removed net XA25: U8.P120, U9.16
- removed net XA26: U8.P118, U9.17
- removed net XA27: U8.P116, U9.18
- removed net XA28: U8.P114, U9.19
- removed net XA29: U8.P112, U9.20
- removed net XA3: U1.P134, U3.6
- removed net XA30: U8.P104, U9.26
- removed net XA31: U8.P102, U9.27
- removed net XA32: U8.P101, U9.28
- removed net XA33: U8.P100, U9.29
- removed net XA34: U8.P111, U9.30
- removed net XA35: U8.P131, U9.38
- removed net XA36: U8.P138, U9.39
- removed net XA37: U8.P140, U9.40
- removed net XA38: U8.P142, U9.41
- removed net XA39: U8.P105, U9.25
- removed net XA4: U1.P133, U3.7
- removed net XA40: U8.P143, U9.42
- removed net XA41: U8.P139, U9.4
- removed net XA42: U15.P141, U16.3
- removed net XA43: U15.P137, U16.5
- removed net XA44: U15.P134, U16.6
- removed net XA45: U15.P133, U16.7
- removed net XA46: U15.P120, U16.16
- removed net XA47: U15.P118, U16.17
- removed net XA48: U15.P116, U16.18
- removed net XA49: U15.P114, U16.19
- removed net XA5: U1.P120, U3.16
- removed net XA50: U15.P112, U16.20
- removed net XA51: U15.P104, U16.26
- removed net XA52: U15.P102, U16.27
- removed net XA53: U15.P101, U16.28
- removed net XA54: U15.P100, U16.29
- removed net XA55: U15.P111, U16.30
- removed net XA56: U15.P131, U16.38
- removed net XA57: U15.P138, U16.39
- removed net XA58: U15.P140, U16.40
- removed net XA59: U15.P142, U16.41
- removed net XA6: U1.P118, U3.17
- removed net XA60: U15.P105, U16.25
- removed net XA61: U15.P143, U16.42
- removed net XA62: U15.P139, U16.4
- removed net XA63: U22.P141, U23.3
- removed net XA64: U22.P137, U23.5
- removed net XA65: U22.P134, U23.6
- removed net XA66: U22.P133, U23.7
- removed net XA67: U22.P120, U23.16
- removed net XA68: U22.P118, U23.17
- removed net XA69: U22.P116, U23.18
- removed net XA7: U1.P116, U3.18
- removed net XA70: U22.P114, U23.19
- removed net XA71: U22.P112, U23.20
- removed net XA72: U22.P104, U23.26
- removed net XA73: U22.P102, U23.27
- removed net XA74: U22.P101, U23.28
- removed net XA75: U22.P100, U23.29
- removed net XA76: U22.P111, U23.30
- removed net XA77: U22.P131, U23.38
- removed net XA78: U22.P138, U23.39
- removed net XA79: U22.P140, U23.40
- removed net XA8: U1.P114, U3.19
- removed net XA80: U22.P142, U23.41
- removed net XA81: U22.P105, U23.25
- removed net XA82: U22.P143, U23.42
- removed net XA83: U22.P139, U23.4
- removed net XA9: U1.P112, U3.20
- removed net XD0: U1.P132, U3.9
- removed net XD1: U1.P127, U3.10
- removed net XD10: U8.P124, U9.13
- removed net XD11: U8.P123, U9.14
- removed net XD12: U8.P115, U9.31
- removed net XD13: U8.P117, U9.32
- removed net XD14: U8.P119, U9.35
- removed net XD15: U8.P126, U9.36
- removed net XD16: U15.P132, U16.9
- removed net XD17: U15.P127, U16.10
- removed net XD18: U15.P124, U16.13
- removed net XD19: U15.P123, U16.14
- removed net XD2: U1.P124, U3.13
- removed net XD20: U15.P115, U16.31
- removed net XD21: U15.P117, U16.32
- removed net XD22: U15.P119, U16.35
- removed net XD23: U15.P126, U16.36
- removed net XD24: U22.P132, U23.9
- removed net XD25: U22.P127, U23.10
- removed net XD26: U22.P124, U23.13
- removed net XD27: U22.P123, U23.14
- removed net XD28: U22.P115, U23.31
- removed net XD29: U22.P117, U23.32
- removed net XD3: U1.P123, U3.14
- removed net XD30: U22.P119, U23.35
- removed net XD31: U22.P126, U23.36
- removed net XD4: U1.P115, U3.31
- removed net XD5: U1.P117, U3.32
- removed net XD6: U1.P119, U3.35
- removed net XD7: U1.P126, U3.36
- removed net XD8: U8.P132, U9.9
- removed net XD9: U8.P127, U9.10
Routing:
- net 3.3V2: track 288.5 -> 0.00 mm, vias 19 -> 0
- net 3.3V3: track 288.5 -> 0.00 mm, vias 19 -> 0
- net 3.3V: track 288.5 -> 0.00 mm, vias 19 -> 0
- net 3.3V1: track 288.5 -> 0.00 mm, vias 19 -> 0
- net 5V: track 233.3 -> 0.00 mm, vias 1 -> 0
- net 5V3: track 233.3 -> 0.00 mm, vias 1 -> 0
- net 5V1: track 233.3 -> 0.00 mm, vias 1 -> 0
- net 5V2: track 233.3 -> 0.00 mm, vias 1 -> 0
- net GND2: track 149.1 -> 0.00 mm, vias 25 -> 0
- net GND3: track 149.1 -> 0.00 mm, vias 25 -> 0
- net GND1: track 149.1 -> 0.00 mm, vias 25 -> 0
- net GND: track 149.1 -> 0.00 mm, vias 25 -> 0
- net L-OUT2: track 112.9 -> 0.00 mm
- net L-OUT1: track 112.9 -> 0.00 mm
- net L-OUT3: track 112.9 -> 0.00 mm
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- removed copper zone on layer 1, net GND
- removed copper zone on layer 16, net GND
- removed copper zone on layer 1, net GND1
- removed copper zone on layer 16, net GND1
- removed copper zone on layer 1, net GND2
- removed copper zone on layer 16, net GND2
- removed copper zone on layer 1, net GND3
- removed copper zone on layer 16, net GND3
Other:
- board text removed: "(C)2015 ZX-Uno Team http://www.zxuno.com"
- board text removed: "1"
- board text removed: "AUDIO"
- board text removed: "C1"
- board text removed: "C10"
- board text removed: "C11"
- board text removed: "C12"
- board text removed: "C13"
- board text removed: "C14"
- board text removed: "C15"
- board text removed: "C16"
- board text removed: "C17"
- board text removed: "C18"
- board text removed: "C19"
- board text removed: "C2"
- board text removed: "C20"
- board text removed: "C21"
- board text removed: "C22"
- board text removed: "C23"
- board text removed: "C24"
- board text removed: "C25"
- board text removed: "C26"
- board text removed: "C27"
- board text removed: "C28"
- board text removed: "C29"
- board text removed: "C3"
- board text removed: "C30"
- board text removed: "C31"
- board text removed: "C32"
- board text removed: "C33"
- board text removed: "C34"
- board text removed: "C35"
- board text removed: "C36"
- board text removed: "C4"
- board text removed: "C5"
- board text removed: "C6"
- board text removed: "C7"
- board text removed: "C8"
- board text removed: "C9"
- board text removed: "CVBS"
- board text removed: "D1"
- board text removed: "D2"
- board text removed: "D3"
- board text removed: "D4"
- board text removed: "D5"
- board text removed: "EAR"
- board text removed: "J10"
- board text removed: "J11"
- board text removed: "J12"
- board text removed: "J16"
- board text removed: "JOY"
- board text removed: "JTAG"
- board text removed: "L1"
- board text removed: "L2"
- board text removed: "L3"
- board text removed: "PS/2"
- board text removed: "PWCON"
- board text removed: "PWUSB"
- board text removed: "R1"
- board text removed: "R10"
- board text removed: "R11"
- board text removed: "R12"
- board text removed: "R13"
- board text removed: "R14"
- board text removed: "R15"
- board text removed: "R16"
- board text removed: "R17"
- board text removed: "R18"
- board text removed: "R19"
- board text removed: "R2"
- board text removed: "R20"
- board text removed: "R21"
- board text removed: "R22"
- board text removed: "R23"
- board text removed: "R24"
- board text removed: "R25"
- board text removed: "R26"
- board text removed: "R27"
- board text removed: "R28"
- board text removed: "R29"
- board text removed: "R3"
- board text removed: "R30"
- board text removed: "R31"
- board text removed: "R32"
- board text removed: "R4"
- board text removed: "R5"
- board text removed: "R6"
- board text removed: "R7"
- board text removed: "R8"
- board text removed: "R9"
- board text removed: "RGB"
- board text removed: "RST"
- board text removed: "SW"
- board text removed: "T1"
- board text removed: "U1"
- board text removed: "U2"
- board text removed: "U3"
- board text removed: "U4"
- board text removed: "U5"
- board text removed: "U6"
- board text removed: "U7"
- board text removed: "Y1"
- board text removed: "Y2"
- board text removed: "v4.1"
